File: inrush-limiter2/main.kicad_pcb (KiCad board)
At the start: 2 copper layers, 32 parts, among them K1 RELAY_2RT, P1 CONN_01X04, P2 CONN_01X02, Q1 2N3904, Q2 PN2222A, T1 TRANSFO, U1 LM393, U2 50 ohm NTC

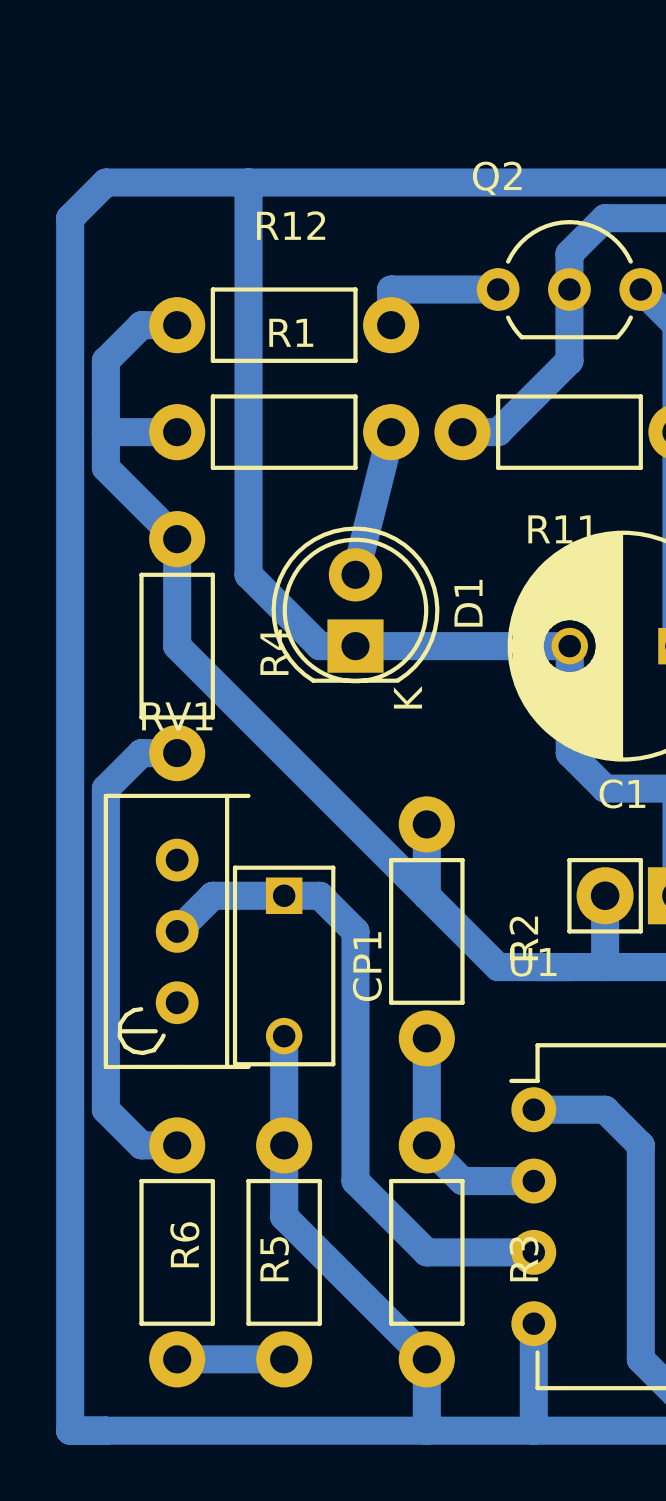
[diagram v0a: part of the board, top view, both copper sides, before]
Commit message: improve traces
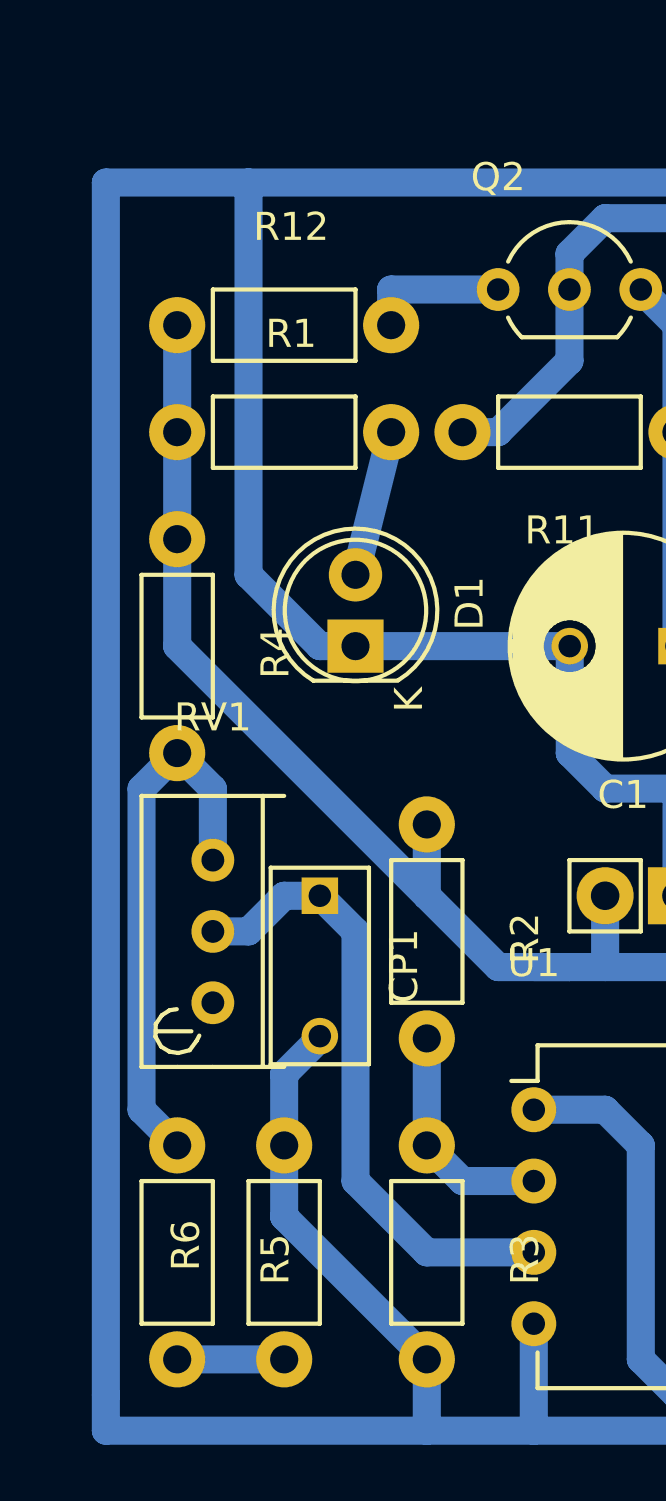
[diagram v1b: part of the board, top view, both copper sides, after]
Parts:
- moved CP1 1.27 mm to (121.9, 76.2)
- moved RV1 1.27 mm to (118.1, 80.0)
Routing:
- net +5V: track 89.6 -> 84.2 mm
- net GND: track 248.3 -> 245.7 mm
- net Net-(R4-Pad2): track 17.6 -> 19.4 mm
- net Net-(CP1-Pad1): track 23.7 -> 22.4 mm
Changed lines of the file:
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@@
   (general
     (links 58)
-    (no_connects 5)
+    (no_connects 4)
     (area 110.105 9.824899 205.148001 96.28099)
     (thickness 1.6)
     (drawings 0)
-    (tracks 165)
+    (tracks 162)
     (zones 0)
     (modules 32)
@@
   )
   (module Capacitors_ThroughHole:C_Rect_L7_W3.5_P5 (layer F.Cu)
-    (at 120.65 76.2 270)
+    (at 121.92 76.2 270)
     (descr "Film Capacitor Length 7mm x Width 3.5mm, Pitch 5mm")
     (tags Capacitor)
@@
   )
   (module Potentiometers:Potentiometer_Bourns_3296W_3-8Zoll_Inline_ScrewUp (layer F.Cu)
-    (at 116.84 80.01)
+    (at 118.11 80.01)
     (descr "3296, 3/8, Square, Trimpot, Trimming, Potentiometer, Bourns")
     (tags "3296, 3/8, Square, Trimpot, Trimming, Potentiometer, Bourns")
@@
   (segment (start 142.24202 69.85) (end 142.24254 69.85052) (width 1) (layer B.Cu) (net 1) (status 30))
   (segment (start 138.43 69.84798) (end 138.43254 69.85052) (width 1) (layer B.Cu) (net 1) (status 30))
+  (segment (start 114.3 50.8) (end 114.3 93.98) (width 1) (layer B.Cu) (net 2))
+  (segment (start 114.3 93.98) (end 114.3 95.25) (width 1) (layer B.Cu) (net 2))
+  (segment (start 121.92 81.2) (end 121.92 81.28) (width 1) (layer B.Cu) (net 2) (status C00000))
+  (segment (start 121.92 81.28) (end 120.65 82.55) (width 1) (layer B.Cu) (net 2) (status 400000))
+  (segment (start 120.65 82.55) (end 120.65 85.09) (width 1) (layer B.Cu) (net 2) (status 800000))
   (segment (start 134.625 72.385) (end 132.085 72.385) (width 1) (layer B.Cu) (net 2))
-  (segment (start 130.82 71.12) (end 130.82 67.31) (width 1) (layer B.Cu) (net 2) (status 800000))
+  (segment (start 130.82 71.12) (end 130.82 67.31) (width 1) (layer B.Cu) (net 2))
   (segment (start 132.085 72.385) (end 130.82 71.12) (width 1) (layer B.Cu) (net 2))
   (segment (start 135.895 72.385) (end 134.625 72.385) (width 1) (layer B.Cu) (net 2))
@@
   (segment (start 121.92 67.31) (end 123.19 67.31) (width 1) (layer B.Cu) (net 2) (status 20))
   (segment (start 148.59052 54.60746) (end 148.59052 53.34052) (width 1) (layer B.Cu) (net 2) (status 10))
-  (segment (start 113.03 52.07) (end 113.03 95.25) (width 1) (layer B.Cu) (net 2))
-  (segment (start 114.3 50.8) (end 113.03 52.07) (width 1) (layer B.Cu) (net 2))
   (segment (start 146.05 50.8) (end 119.38 50.8) (width 1) (layer B.Cu) (net 2))
   (segment (start 119.38 50.8) (end 114.3 50.8) (width 1) (layer B.Cu) (net 2))
   (segment (start 148.59052 53.34052) (end 146.05 50.8) (width 1) (layer B.Cu) (net 2))
-  (segment (start 113.03 95.25) (end 114.3 95.25) (width 1) (layer B.Cu) (net 2))
   (segment (start 158.75 93.98) (end 158.75 87.63) (width 1) (layer B.Cu) (net 2))
   (segment (start 139.7 88.9) (end 137.16 88.9) (width 1) (layer B.Cu) (net 2) (status 20))
@@
   (segment (start 138.43 91.44) (end 137.16 91.44) (width 1) (layer B.Cu) (net 2) (status 20))
   (segment (start 125.73 95.25) (end 114.3 95.25) (width 1) (layer B.Cu) (net 2))
-  (segment (start 114.3 95.25) (end 113.03 95.25) (width 1) (layer B.Cu) (net 2))
   (segment (start 129.54 91.44) (end 129.54 95.25) (width 1) (layer B.Cu) (net 2) (status 10))
   (segment (start 125.73 95.25) (end 125.73 92.71) (width 1) (layer B.Cu) (net 2) (status 20))
@@
   (segment (start 148.59052 54.60746) (end 148.58746 54.60746) (width 1) (layer B.Cu) (net 2) (status 30))
   (segment (start 146.05 69.84694) (end 146.04746 69.84948) (width 1) (layer B.Cu) (net 2) (status 30))
-  (segment (start 120.73 81.2) (end 120.65 81.2) (width 1) (layer B.Cu) (net 2) (status 30))
-  (segment (start 120.65 81.2) (end 120.65 85.09) (width 1) (layer B.Cu) (net 2) (status 30))
+  (segment (start 122 81.2) (end 121.92 81.2) (width 1) (layer B.Cu) (net 2) (status 30))
   (segment (start 125.69 92.67) (end 125.73 92.71) (width 1) (layer B.Cu) (net 2) (status 30))
   (segment (start 123.19254 67.31052) (end 123.19 67.30798) (width 1) (layer B.Cu) (net 2) (status 30))
@@
   (segment (start 142.24 90.17) (end 142.24 92.71) (width 1) (layer B.Cu) (net 7) (status 10))
   (segment (start 142.24052 83.81948) (end 142.24 83.82) (width 1) (layer B.Cu) (net 7) (status 30))
-  (segment (start 116.84 71.12) (end 115.57 71.12) (width 1) (layer B.Cu) (net 8))
-  (segment (start 115.57 85.09) (end 116.84 85.09) (width 1) (layer B.Cu) (net 8))
-  (segment (start 114.3 83.82) (end 115.57 85.09) (width 1) (layer B.Cu) (net 8))
-  (segment (start 114.3 72.39) (end 114.3 83.82) (width 1) (layer B.Cu) (net 8))
-  (segment (start 115.57 71.12) (end 114.3 72.39) (width 1) (layer B.Cu) (net 8))
+  (segment (start 116.84 71.12) (end 115.57 72.39) (width 1) (layer B.Cu) (net 8) (status 400000))
+  (segment (start 115.57 83.82) (end 116.84 85.09) (width 1) (layer B.Cu) (net 8) (status 800000))
+  (segment (start 115.57 72.39) (end 115.57 83.82) (width 1) (layer B.Cu) (net 8))
+  (segment (start 118.11 74.93) (end 118.11 72.39) (width 1) (layer B.Cu) (net 8) (status 400000))
+  (segment (start 118.11 72.39) (end 116.84 71.12) (width 1) (layer B.Cu) (net 8) (status 800000))
   (segment (start 170.18 76.2) (end 163.83 76.2) (width 2.5) (layer B.Cu) (net 9) (status 30))
   (segment (start 186.69 36.83) (end 186.52998 35.39998) (width 0.75) (layer B.Cu) (net 11) (status 30))
@@
   (segment (start 125.73 85.09) (end 125.73 81.28) (width 1) (layer B.Cu) (net 19) (status 30))
   (segment (start 120.65 92.71) (end 116.84 92.71) (width 1) (layer B.Cu) (net 20) (status 30))
-  (segment (start 120.65 76.2) (end 118.11 76.2) (width 1) (layer B.Cu) (net 21))
-  (segment (start 118.11 76.2) (end 116.84 77.47) (width 1) (layer B.Cu) (net 21))
+  (segment (start 121.92 76.2) (end 120.65 76.2) (width 1) (layer B.Cu) (net 21) (status 400000))
+  (segment (start 119.38 77.47) (end 118.11 77.47) (width 1) (layer B.Cu) (net 21) (status 800000))
+  (segment (start 120.65 76.2) (end 119.38 77.47) (width 1) (layer B.Cu) (net 21))
   (segment (start 123.19 77.47) (end 123.19 86.36) (width 1) (layer B.Cu) (net 21))
   (segment (start 121.92 76.2) (end 123.19 77.47) (width 1) (layer B.Cu) (net 21))
   (segment (start 125.73 88.9) (end 129.54 88.9) (width 1) (layer B.Cu) (net 21) (status 20))
   (segment (start 123.19 86.36) (end 125.73 88.9) (width 1) (layer B.Cu) (net 21))
-  (segment (start 121.92 76.2) (end 120.65 76.2) (width 1) (layer B.Cu) (net 21) (status 20))
-  (segment (start 132.08 76.2) (end 132.08 78.74) (width 1) (layer B.Cu) (net 22) (status 400000))
+  (segment (start 121.92 76.2) (end 121.92 76.2) (width 1) (layer B.Cu) (net 21) (status 20))
+  (segment (start 116.84 63.5) (end 116.84 59.69) (width 1) (layer B.Cu) (net 22) (status C00000))
+  (segment (start 116.84 59.69) (end 116.84 55.88) (width 1) (layer B.Cu) (net 22) (status C00000))
+  (segment (start 132.08 76.2) (end 132.08 78.74) (width 1) (layer B.Cu) (net 22))
   (segment (start 129.54 78.74) (end 130.81 78.74) (width 1) (layer B.Cu) (net 22))
   (segment (start 125.73 73.66) (end 125.73 76.2) (width 1) (layer B.Cu) (net 22))
@@
   (segment (start 132.08 78.74) (end 137.16 78.74) (width 1) (layer B.Cu) (net 22))
   (segment (start 116.84 63.5) (end 116.84 67.31) (width 1) (layer B.Cu) (net 22) (status 10))
-  (segment (start 116.84 59.69) (end 114.3 59.69) (width 1) (layer B.Cu) (net 22) (status 10))
-  (segment (start 116.84 55.88) (end 115.57 55.88) (width 1) (layer B.Cu) (net 22) (status 10))
-  (segment (start 114.3 60.96) (end 116.84 63.5) (width 1) (layer B.Cu) (net 22) (status 20))
-  (segment (start 114.3 57.15) (end 114.3 59.69) (width 1) (layer B.Cu) (net 22))
-  (segment (start 114.3 59.69) (end 114.3 60.96) (width 1) (layer B.Cu) (net 22))
-  (segment (start 115.57 55.88) (end 114.3 57.15) (width 1) (layer B.Cu) (net 22))
   (segment (start 116.84 67.31) (end 125.73 76.2) (width 1) (layer B.Cu) (net 22))
   (segment (start 147.32 76.2) (end 149.86 76.2) (width 1) (layer B.Cu) (net 22) (status 10))
